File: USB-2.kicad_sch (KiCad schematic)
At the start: 55 parts, among them J6 USB_C_Receptacle_USB2.0_16P, J7 USB_A_Stacked, J8 USB_A_Stacked, U10 USBLC6-2P6, U11 USBLC6-2P6, U12 USBLC6-2P6, U13 USBLC6-2P6, U5 USB2514B-I/M2, U6 FSUSB42MUX, U7 MIC2026-1xM, U8 MIC2026-1xM, U9 USBLC6-2P6, Y1 24MHz

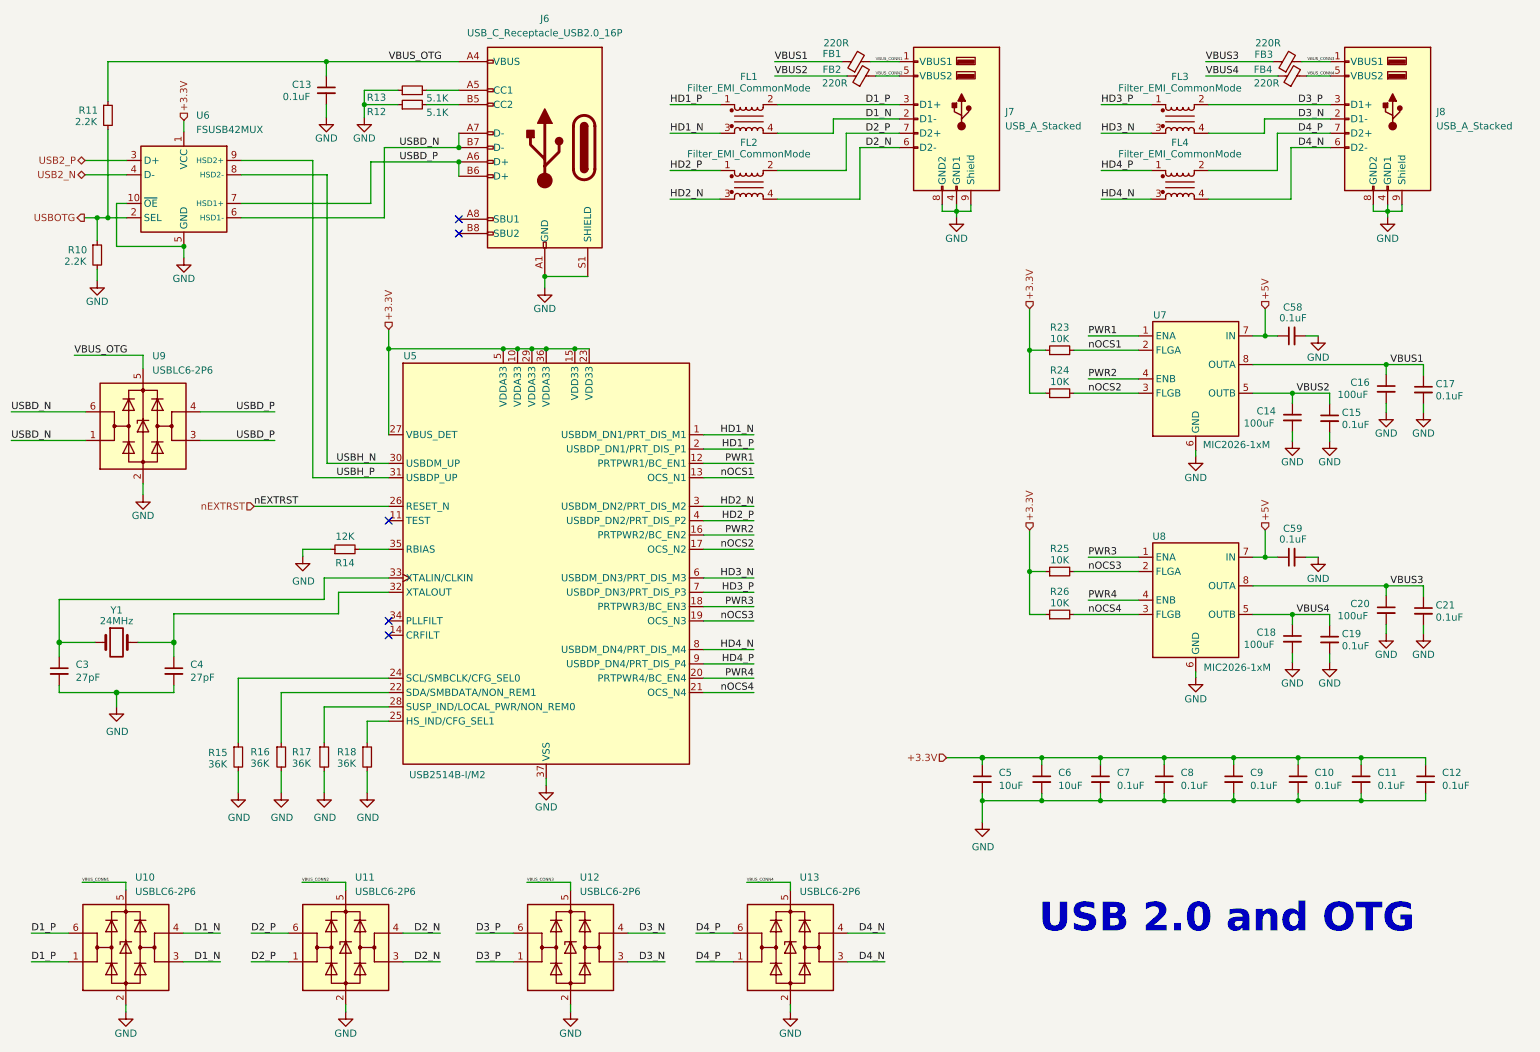
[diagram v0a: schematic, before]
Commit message: More stuff idk
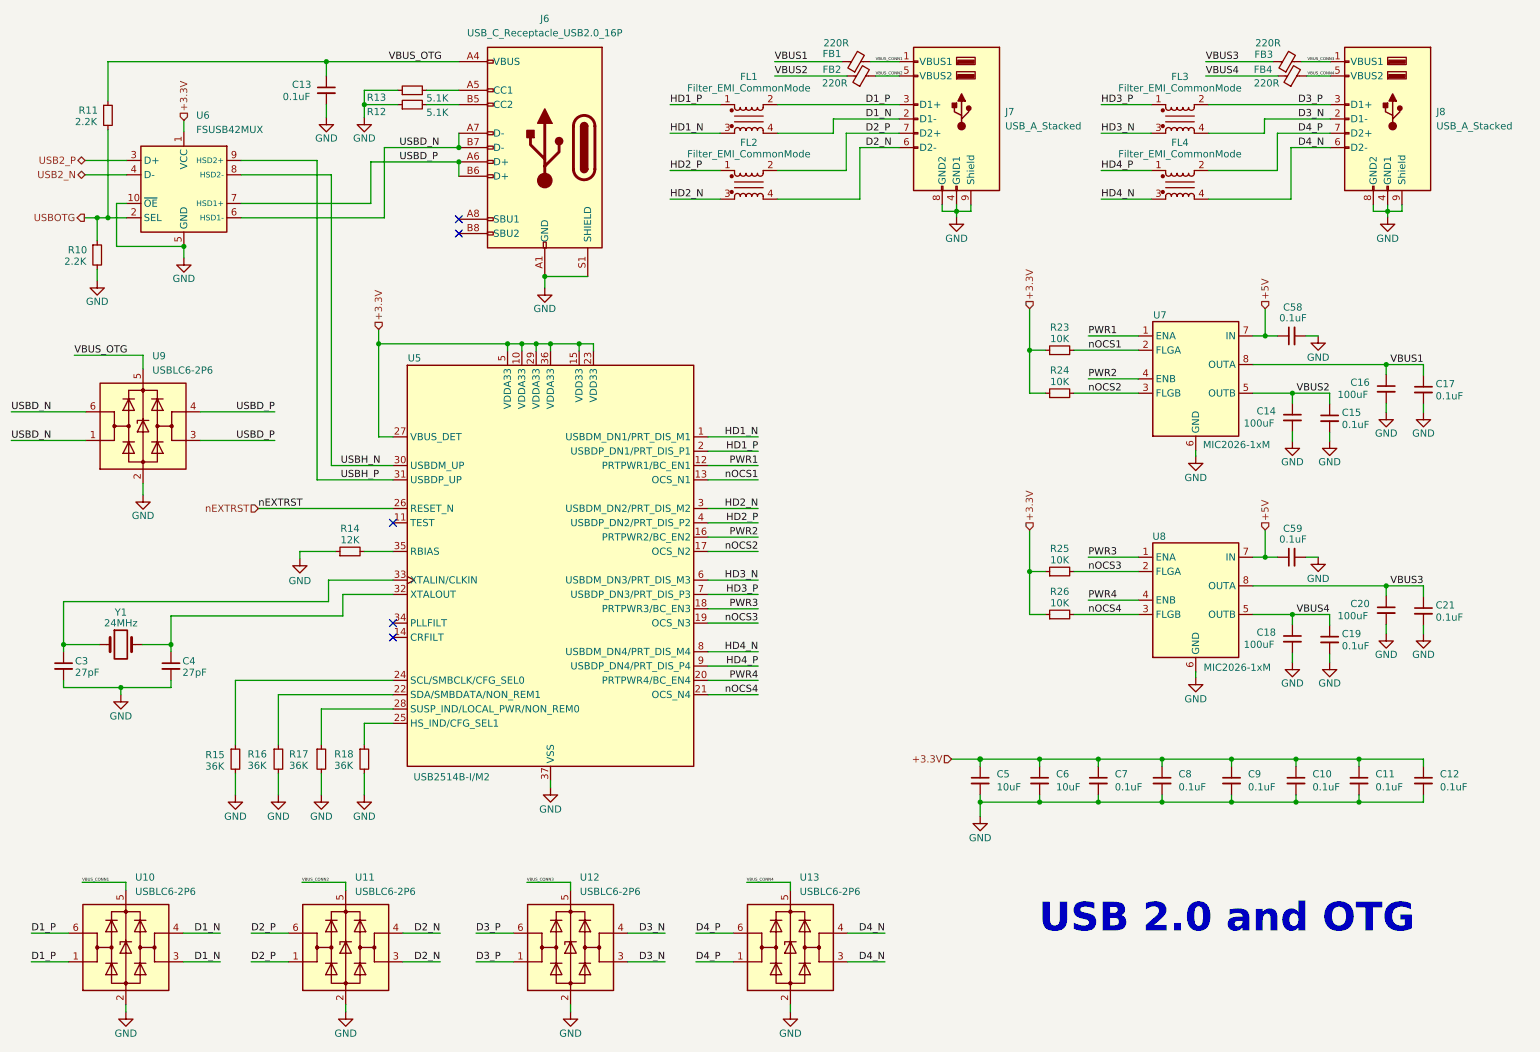
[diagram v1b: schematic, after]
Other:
- moved on the sheet: C3, C4, R14, R15, R16, R17, R18, U5, Y1
